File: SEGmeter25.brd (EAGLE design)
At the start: 104.1 x 83.8 mm, 134 parts, among them IC1 DS1307, IC2 LD1117S50, IC3 LD1117S33, IC4 XBEE, IC5 ATmega328, IC6 MCP1541, IC7 MCP3208, J1 Short 12V, J10 3.5mm, J11 3.5mm, J12 Relays, J13 3.5mm, J14 Star ground, J15 3.5mm, J16 Arduino-compatible headers, J17 3.5mm, J18 3.5mm, J2 1-Wire, J3 ISP, J4 Power, J5 Comms, J6 MICROSD, J7 Sensor 5V, J8 3.5mm, J9 3.5mm, Q1 32768 Hz, Q2 16 MHz, Q3 2N7002, Q4 2N7002, Q5 2N7002

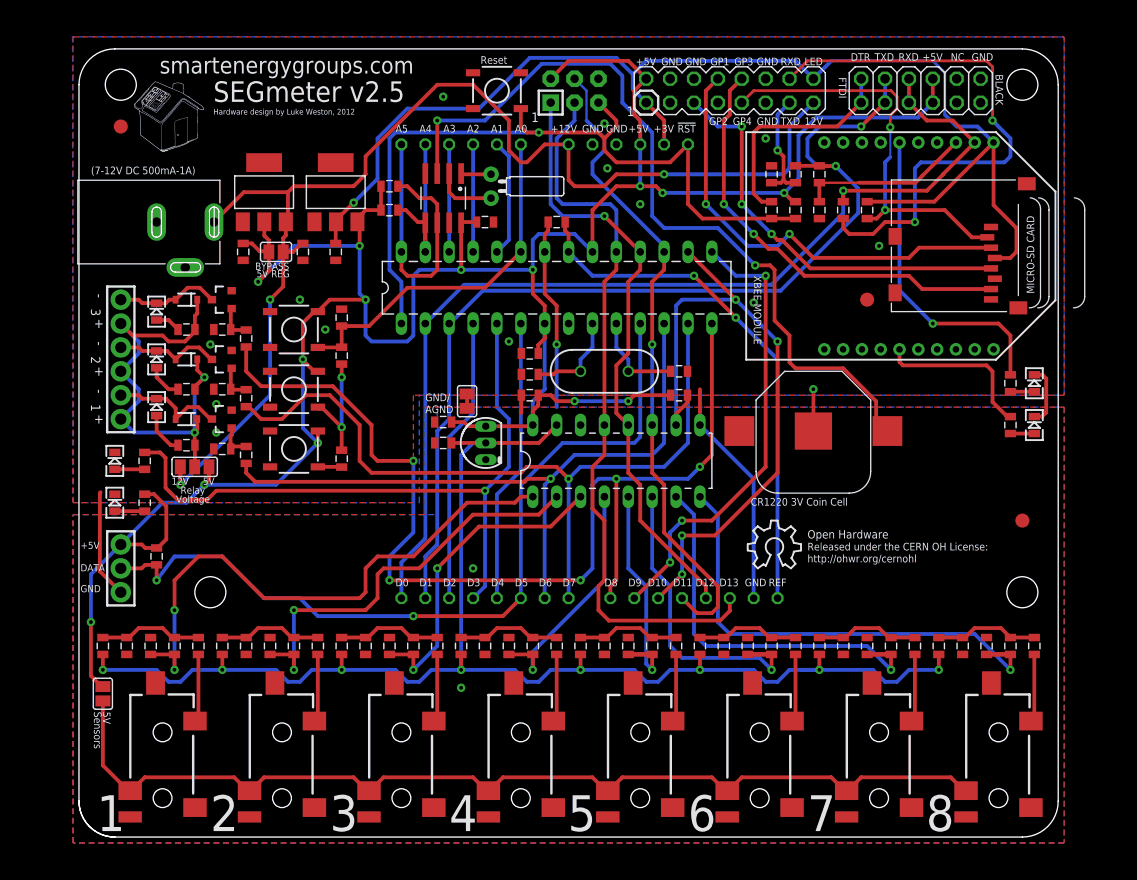
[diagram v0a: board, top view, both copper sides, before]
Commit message: foo
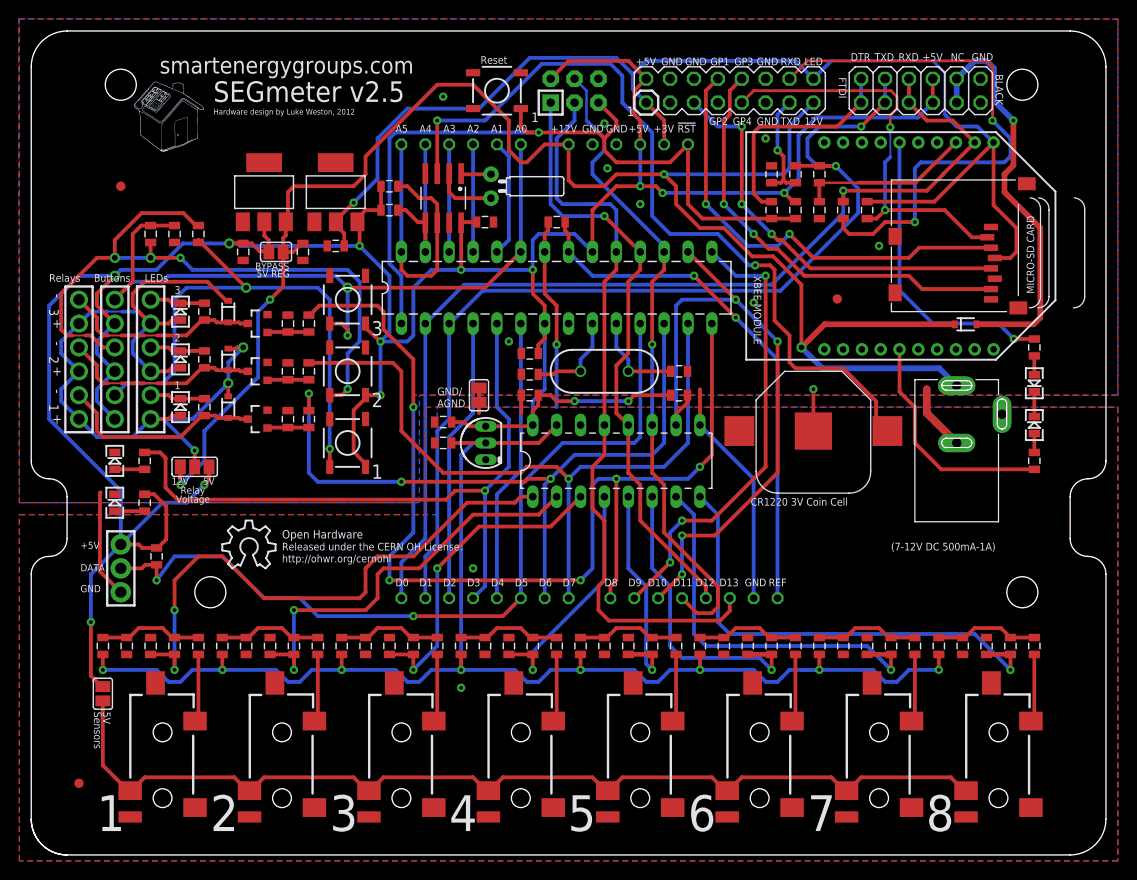
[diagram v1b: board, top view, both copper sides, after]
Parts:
- removed JP5, JP6, JP7: FIDUCIAL1.5X3, SparkFun:FIDUCIAL-1.5X3
- added D4: 1N4148, SparkFun:SOD-323
- added FID1, FID2, FID3: FIDUCIAL, adafruit:FIDUCIAL_1MM
- added J19, J20: 3.5mm, SparkFun:AUDIO-JACK-3.5MM-SMD
- J12: value Relays -> 3.5mm; device con-phoenix-254:6POL254 -> SparkFun:AUDIO-JACK-3.5MM-SMD
- J14: value Star ground -> Relays; device freetronics-luke:SJ -> con-phoenix-254:6POL254
- J16: value Arduino-compatible headers -> Star ground; device Arduino-Various:NO-OUTLINE-OCTAGONAL-NOTEXT -> freetronics-luke:SJ
- J18: value 3.5mm -> Arduino-compatible headers; device SparkFun:AUDIO-JACK-3.5MM-SMD -> Arduino-Various:NO-OUTLINE-OCTAGONAL-NOTEXT
- J7: value Sensor 5V -> Buttons; device freetronics-luke:SJ -> con-phoenix-254:6POL254
- J8: value 3.5mm -> Relay LEDs; device SparkFun:AUDIO-JACK-3.5MM-SMD -> con-phoenix-254:6POL254
- J9: value 3.5mm -> Sensor 5V; device SparkFun:AUDIO-JACK-3.5MM-SMD -> freetronics-luke:SJ
- LED1: value Status -> RSSI
- LED2: value Power -> Assoc
- LED3: value RSSI -> Status
- LED4: value Assoc -> Power
- R1, R2: value 1k -> 4k7
- R11, R17, R7, R8: value 10k -> 1k
- R12: value 3k3 -> 1k
- R13, R14, R9: value 1k -> 10k
- R15: value 10k -> 220k
- R16: value 2k2 -> 3k3
- R21: value 220k -> 1k
- R22: value 1k -> 2k2
- R30, R31: value 3k3 -> 220k
- R33, R34: value 220k -> 3k3
- R5, R6: value 4k7 -> 10k
- moved LED1 98.1 mm to (101.6, 48.3), turned to 270 degrees
- moved LED2 98.1 mm to (101.6, 43.8)
- moved LED3 98.1 mm to (3.81, 40.0)
- moved LED4 98.1 mm to (3.81, 35.6)
- moved R15 89.1 mm to (2.54, 20.3), turned to 270 degrees
- moved J4 88.3 mm to (93.3, 41.9), turned to 0 degrees
- moved D1 83.5 mm to (94.3, 54.5), turned to 0 degrees
- moved R11 81.3 mm to (6.99, 40.0)
- moved R17 80.9 mm to (10.2, 20.3)
- moved R5 77.3 mm to (76.2, 66.7), turned to 270 degrees
- moved J18 61.5 mm to (62.2, 50.8)
- moved J12 58.4 mm to (34.3, 0.64)
- moved U$1 55.9 mm to (15.2, 28.6)
- moved R34 53.5 mm to (13.3, 55.9), turned to 90 degrees
- moved R13 52.0 mm to (76.2, 70.5), turned to 90 degrees
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- renumbered JP1 to H1, JP2 to H2, JP3 to H3, JP4 to H4
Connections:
- removed net N$24: LED5.A, R30.1
- removed net N$25: R12.2, S2.1
- removed net N$27: LED6.A, R31.1
- removed net N$31: R12.1, R13.2, S3.1
- removed net N$58: LED7.A, R32.1
- removed net N$72: D1.1, D2.1, D3.1, J12.1, J12.3, J12.5, R30.2, R31.2, R32.2, SJ1.2
- new net BUTTON1: J7.2, R16.2, S2.1
- new net BUTTON2: J7.4, R16.1, R19.2, S3.1
- new net N$3: D1.2, J5.10, J5.9
- new net RELAY1LED: J8.2, LED5.C, R32.2
- new net RELAY2LED: J8.4, LED6.C, R33.2
- new net RELAY3LED: J8.6, LED7.C, R34.2
- new net RELAY_VOLTAGE: D2.1, D3.1, D4.1, J14.1, J14.3, J14.5, J8.1, J8.3, J8.5, LED5.A, LED6.A, LED7.A, SJ1.2
- net !ADC1_CS: now also J18.10; no longer J16.10
- net !ADC2_CS: now also J18.9; no longer J16.9
- net !GPIO_CS: now also R9.1; no longer R11.1
- net !RESET: now also J18.RESET, R5.2; no longer J16.RESET, R7.2
- net +12V: now also D1.1, J18.VIN; no longer J16.VIN
- net +3V3: now also J18.3V3, R9.2; no longer J16.3V3, R11.2
- net +5V: now also J18.5V, J7.1, J7.3, J7.5, J9.2, R1.2, R12.2, R5.1; no longer J16.5V, J7.2, R4.2, R5.2, R7.1
- net 1WIRE: now also J18.5, R3.1; no longer J16.5, R5.1
- net 3.3VTXD: now also R4.2, R6.1; no longer R6.2, R8.1
- net A1: now also J18.A_1; no longer J16.A_1
- net A2: now also J18.A_2; no longer J16.A_2
- net A3: now also J18.A_3; no longer J16.A_3
- net AGND: now also J12.SLEEVE, J16.2, J19.SLEEVE, J20.SLEEVE, R18.1, R30.1; no longer J14.2, J18.SLEEVE, J8.SLEEVE, J9.SLEEVE, R20.1, R33.1
- net AREF: now also J18.AREF; no longer J16.AREF
- net BUTTONS: now also J18.A_0, J7.6, R19.1, R22.2; no longer J16.A_0, R13.1, R16.2
- net GND: now also J16.1, J18.GND0, J18.GND1, J18.GND2, R14.2, R22.1, R6.2; no longer J14.1, J16.GND0, J16.GND1, J16.GND2, R16.1, R17.2, R8.2
- net MISO: now also J18.12; no longer J16.12
- net MOSI: now also J18.11; no longer J16.11
- net N$1: now also LED4.A, R12.1; no longer LED2.A, R2.1
- net N$18: now also D2.2, J14.2, R32.1; no longer D1.2, J12.2, LED5.C
- net N$2: now also LED3.A, R11.1; no longer LED1.A, R1.1
- net N$26: now also D3.2, J14.4, R33.1; no longer D2.2, J12.4, LED6.C
- net N$30: now also J20.TIP; no longer J18.TIP
- net N$4: now also R7.1; no longer R9.1
- net N$40: now also D4.2, J14.6, R34.1; no longer D3.2, J12.6, LED7.C
- net N$41: now also J19.TIP; no longer J17.TIP
- net N$42: now also J10.TIP; no longer J8.TIP
- net N$44: now also J11.TIP; no longer J9.TIP
- net N$45: now also J17.TIP; no longer J15.TIP
- net N$46: now also J12.RING, J19.RING, J20.RING, J9.1; no longer J18.RING, J7.1, J8.RING, J9.RING
- net N$47: now also J15.TIP; no longer J13.TIP
- net N$48: now also J13.TIP; no longer J11.TIP
- net N$49: now also J12.TIP; no longer J10.TIP
- net N$5: now also R8.1; no longer R10.1
- net N$50: now also R15.1, R17.2, R18.2; no longer R18.1, R19.2, R20.2
- net N$54: now also R31.1; no longer R34.1
- net N$55: now also R20.1, R21.2; no longer R21.1, R22.2
- net N$57: now also R30.2; no longer R33.2
- net N$6: now also LED2.A, R8.2; no longer LED4.A, R10.2
- net N$60: now also R21.1; no longer R22.1
- net N$7: now also LED1.A, R7.2; no longer LED3.A, R9.2
- net N$70: now also R17.1; no longer R19.1
- net RELAY1: now also J18.6; no longer J16.6
- net RELAY2: now also J18.7; no longer J16.7
- net RELAY3: now also J18.8; no longer J16.8
- net RXD: now also J18.0_RX, R10.2; no longer J16.0_RX, R14.2
- net SCK: now also J18.13; no longer J16.13
- net SCL: now also J18.A_5, R1.1; no longer J16.A_5, R3.1
- net SDA: now also J18.A_4, R2.1; no longer J16.A_4, R4.1
- net SIN: now also R13.1, R14.1; no longer R15.1, R17.1
- net SOUT: now also R10.1; no longer R14.1
- net SPARE: now also J18.2; no longer J16.2
- net SPARE2: now also J18.4; no longer J16.4
- net STATUS_LED: now also J18.3, R11.2; no longer J16.3, R1.2
- net TXD: now also J18.1_TX, R13.2, R4.1; no longer J16.1_TX, R15.2, R6.1
- net V+: now also R15.2, R20.2, R31.2; no longer R18.2, R21.2, R34.2
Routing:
- net RELAY_VOLTAGE: track 0.00 -> 88.5 mm, vias 0 -> 3
- net BUTTON2: track 0.00 -> 73.0 mm, vias 0 -> 4
- net BUTTON1: track 0.00 -> 57.8 mm, vias 0 -> 2
- net +12V: track 127.6 -> 181.2 mm, vias 3 -> 4
- net N$72: track 49.8 -> 0.00 mm, vias 2 -> 0
- net +5V: track 289.0 -> 338.1 mm
- net N$3: track 0.79 -> 44.0 mm, vias 0 -> 1
- net BUTTONS: track 38.5 -> 78.2 mm, vias 0 -> 2
- net N$31: track 12.6 -> 0.00 mm, vias 2 -> 0
- net GND: track 47.1 -> 57.3 mm, vias 14 -> 9
- net N$40: track 11.1 -> 21.1 mm
- net N$26: track 11.3 -> 21.1 mm
- net N$18: track 12.5 -> 22.0 mm
- net N$5: track 17.4 -> 24.5 mm
- net RELAY1LED: track 0.00 -> 5.87 mm
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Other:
- board size 104.1 x 83.8 mm -> 114.3 x 87.6 mm
- board text added: "Buttons"
- board text added: "LEDs"
- board text added: "Relays"
